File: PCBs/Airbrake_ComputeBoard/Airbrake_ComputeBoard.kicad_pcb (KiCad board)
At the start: 2 copper layers, 46.5 x 71.8 mm, 25 parts, among them Q1 PNP, Q2 PNP, Q3 PNP, Q4 PNP

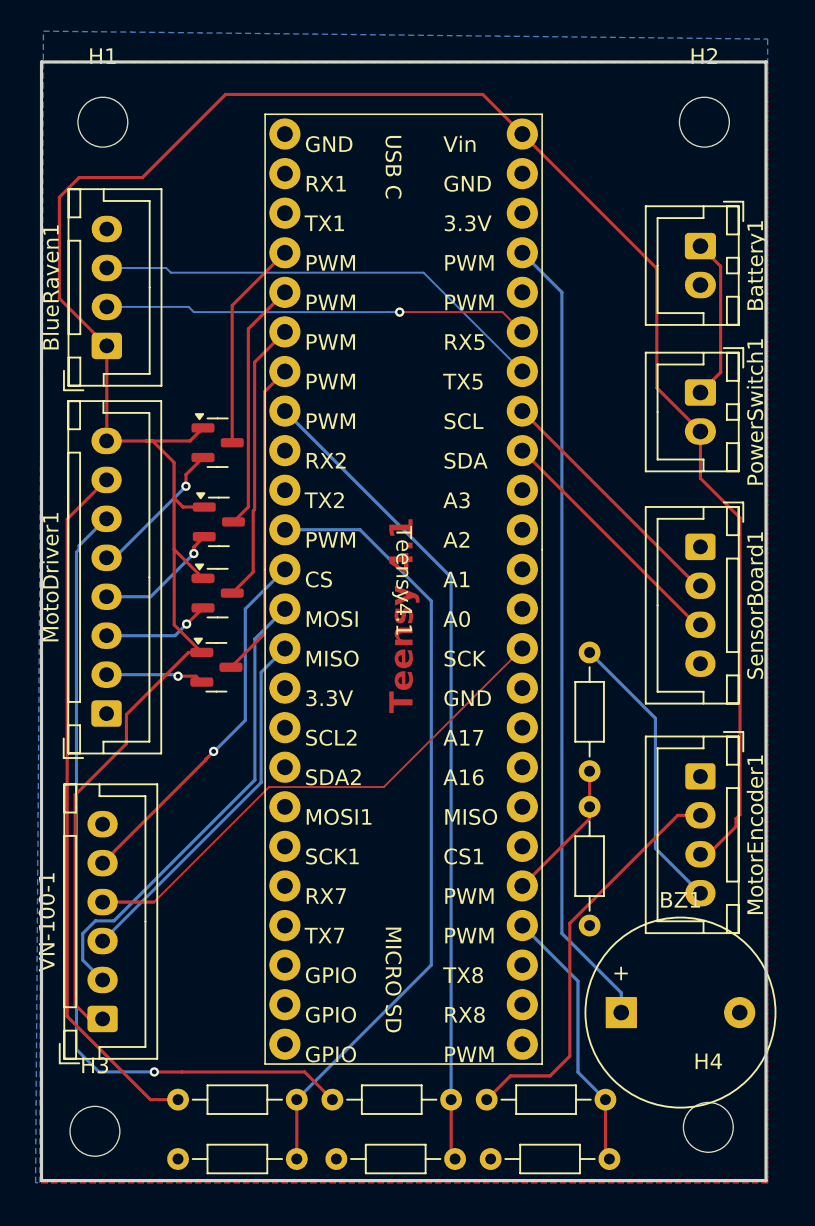
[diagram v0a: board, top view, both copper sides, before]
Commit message: created compute board v1.1
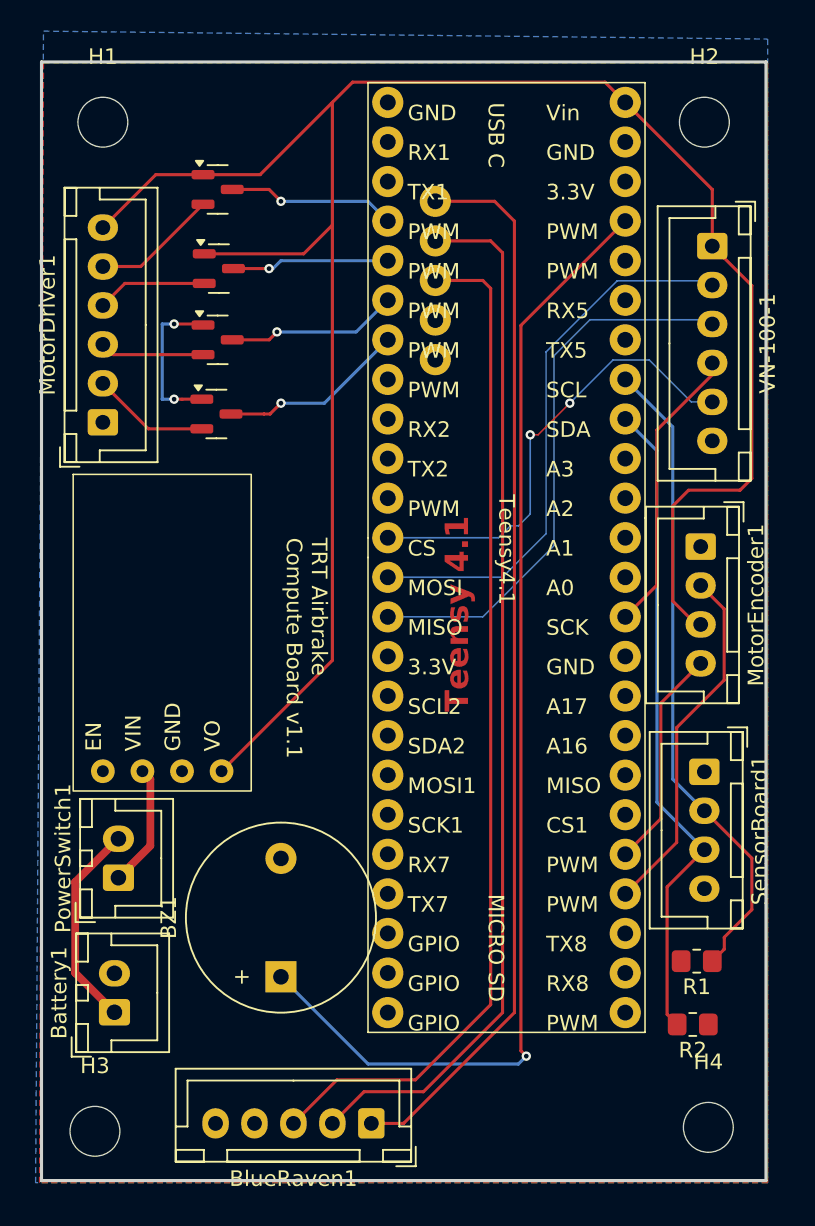
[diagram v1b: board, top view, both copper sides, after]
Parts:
- removed MotoDriver1: Conn_01x08, Connector_JST:JST_XH_B8B-XH-A_1x08_P2.50mm_Vertical
- removed R3, R5, R7: 1.7 kOhm, Resistor_THT:R_Axial_DIN0204_L3.6mm_D1.6mm_P7.62mm_Horizontal
- removed R4, R6, R8: 3.3 kOhm, Resistor_THT:R_Axial_DIN0204_L3.6mm_D1.6mm_P7.62mm_Horizontal
- added Buck_Converter1: ~, Breakout Boards:Buck_Converter, F.Cu at (142.7, 100.3)
- added MotorDriver1: Conn_01x06, Connector_JST:JST_XH_B6B-XH-A_1x06_P2.50mm_Vertical, F.Cu at (138.9, 86.8)
- BlueRaven1: value Conn_01x04 -> Conn_01x05; footprint Connector_JST:JST_XH_B4B-XH-A_1x04_P2.50mm_Vertical -> Connector_JST:JST_XH_B5B-XH-A_1x05_P2.50mm_Vertical
- R1: value 1.7 kOhm -> 3.3kΩ; footprint Resistor_THT:R_Axial_DIN0204_L3.6mm_D1.6mm_P7.62mm_Horizontal -> Resistor_SMD:R_0805_2012Metric_Pad1.20x1.40mm_HandSolder
- R2: value 3.3 kOhm -> 3.3kΩ; footprint Resistor_THT:R_Axial_DIN0204_L3.6mm_D1.6mm_P7.62mm_Horizontal -> Resistor_SMD:R_0805_2012Metric_Pad1.20x1.40mm_HandSolder
- Teensy4.1: footprint Breakout Boards:Teensy_4.1 -> Breakout Boards:Teensy_4.1_USB
- moved VN-100-1 63.2 mm to (178.1, 75.5), turned to -90 degrees
- moved Battery1 61.9 mm to (139.7, 124.7), turned to 90 degrees
- moved BlueRaven1 52.7 mm to (156.2, 131.8), turned to 180 degrees
- moved PowerSwitch1 48.6 mm to (139.9, 116.1), turned to 90 degrees
- moved R1 34.5 mm to (177.1, 121.4), turned to 180 degrees
- moved R2 26.8 mm to (176.8, 125.5)
- moved BZ1 22.0 mm to (150.4, 122.4), turned to 90 degrees
- moved Q1 16.3 mm to (146.2, 86.3)
- moved Q2 16.3 mm to (146.3, 81.5)
- moved Q3 16.3 mm to (146.4, 77.0)
- moved Q4 16.3 mm to (146.3, 71.9)
- moved MotorEncoder1 14.8 mm to (177.3, 94.8)
- moved SensorBoard1 14.4 mm to (177.5, 109.3)
- moved Teensy4.1 6.91 mm to (164.8, 95.5)
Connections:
- net /EN renamed /Stop
- net /F/R renamed /Dir
- BlueRaven1 pad 1: /5v_switch -> /usb_5v
- BlueRaven1 pad 2: /BR-TX -> /D-
- BlueRaven1 pad 3: /BR-RX -> /D+
- MotorEncoder1 pad 2: /A_5v -> /Encoder_A
- MotorEncoder1 pad 3: /5v_switch -> +5V
- MotorEncoder1 pad 4: /B_5v -> /Encoder_B
- PowerSwitch1 pad 1: Net-(Battery1-Pin_1) -> Net-(Buck_Converter1-VIN)
- PowerSwitch1 pad 2: /5v_switch -> Net-(Battery1-Pin_1)
- Q1 pad 3: /5v_switch -> GND
- Q2 pad 3: /5v_switch -> GND
- Q3 pad 3: /5v_switch -> +5V
- Q4 pad 3: /5v_switch -> +5V
- R1 pad 1: /ALM_5v -> /SCL
- R1 pad 2: /ALM_3.3v -> +3.3V
- R2 pad 1: /ALM_3.3v -> +3.3V
- R2 pad 2: GND -> /SDA
- Teensy4.1 pad 10: /ALM_3.3v -> unconnected-(Teensy4.1-PWM-Pad10)
- Teensy4.1 pad 27: /A_3.3v -> /Encoder_A
- Teensy4.1 pad 28: /B_3.3v -> /Encoder_B
- Teensy4.1 pad 47: /5v_switch -> +5V
- Teensy4.1 pad 7: /PG_3.3v -> unconnected-(Teensy4.1-PWM-Pad7)
- VN-100-1 pad 1: /5v_switch -> +5V
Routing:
- net /5v_switch: track 159.0 -> 0.00 mm
- net +5V: track 0.00 -> 134.6 mm
- net /usb_5v: track 0.00 -> 68.5 mm
- net /D-: track 0.00 -> 67.3 mm
- net /D+: track 0.00 -> 65.6 mm
- net /PG_5v: track 52.6 -> 0.00 mm, vias 1 -> 0
- net /PG_3.3v: track 52.5 -> 0.00 mm
- net /ALM_3.3v: track 50.7 -> 0.00 mm
- net /ALM_5v: track 44.8 -> 0.00 mm
- net /BR-RX: track 29.4 -> 0.00 mm
- net /BR-TX: track 27.3 -> 0.00 mm, vias 1 -> 0
- net /A_5v: track 26.3 -> 0.00 mm
- net /SDA: track 16.1 -> 42.2 mm
- net /SCL: track 16.1 -> 41.8 mm
- net /buzzer: track 51.4 -> 74.8 mm, vias 0 -> 1
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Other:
- board text added: "TRT Airbrake Compute Board v1.1"
